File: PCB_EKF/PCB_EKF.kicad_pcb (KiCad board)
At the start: 2 copper layers, 97.8 x 84.6 mm, 41 parts, among them J1 Load, J2 5V, J4 UART, K1 SANYOU_SRD_Form_C, K3 SANYOU_SRD_Form_C, Q1 Q_NMOS_GSD, Q3 Q_NMOS_GSD, SW1 SW_Push_SPDT, U1 INA226_module, U3 YAAJ_BlackPill_Part_Like_SWD_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, U4 TP4056_Module, U5 AMS1117-3.3

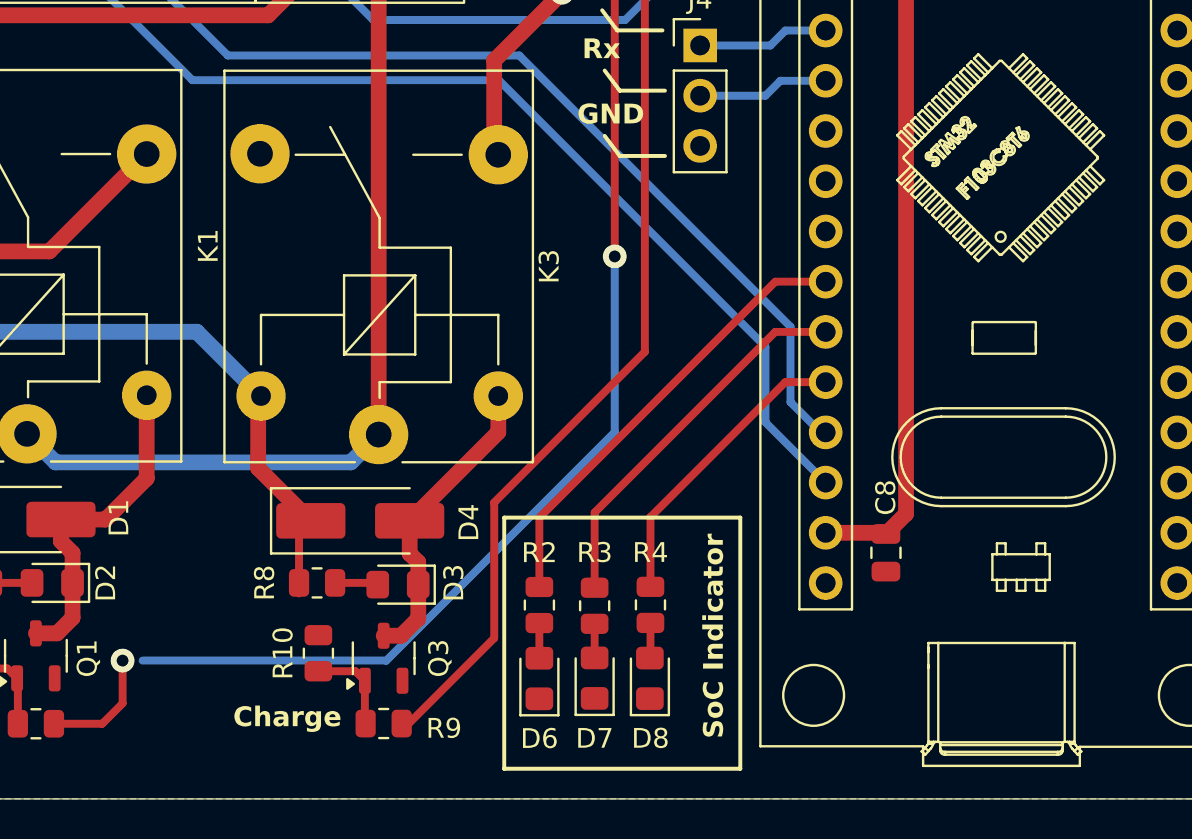
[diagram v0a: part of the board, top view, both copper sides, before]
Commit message: add a lot
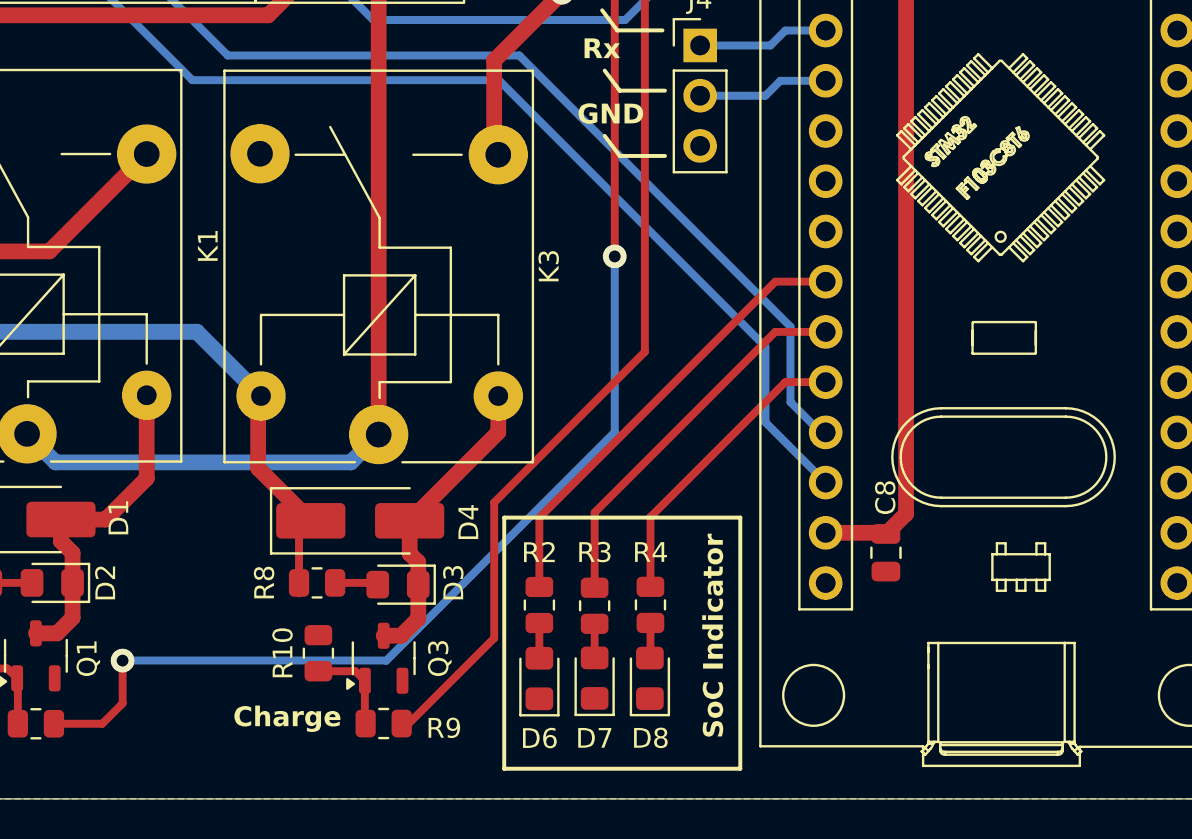
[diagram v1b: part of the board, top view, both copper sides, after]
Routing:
- net CTRL_Load: track 87.8 -> 88.8 mm
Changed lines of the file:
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@@
 			(outputformat 1)
 			(mirror no)
-			(drillshape 1)
+			(drillshape 0)
 			(scaleselection 1)
-			(outputdirectory "")
+			(outputdirectory "Gerber/")
 		)
 	)
@@
 		(fp_arc
 			(start 5.210659 19.015233)
-			(mid 5.273125 18.98719)
+			(mid 5.273123 18.987169)
 			(end 5.341329 18.993348)
 			(stroke
@@
 		(fp_arc
 			(start 6.981719 17.244173)
-			(mid 7.051919 17.214426)
+			(mid 7.051919 17.214488)
 			(end 7.121632 17.245341)
 			(stroke
@@
 		(fp_arc
 			(start 8.464456 19.37686)
-			(mid 8.346161 19.099702)
+			(mid 8.346155 19.099702)
 			(end 8.463393 18.822096)
 			(stroke
@@
 		(fp_arc
 			(start 8.924989 18.360501)
-			(mid 9.075715 18.294215)
+			(mid 9.075715 18.294151)
 			(end 9.227336 18.358376)
 			(stroke
@@
 		(fp_arc
 			(start 9.017838 18.458024)
-			(mid 9.077292 18.432027)
+			(mid 9.077292 18.432091)
 			(end 9.136717 18.458131)
 			(stroke
@@
 		(fp_arc
 			(start 11.989999 48.971818)
-			(mid 11.906797 49.125261)
+			(mid 11.906813 49.12524)
 			(end 11.739999 49.176605)
 			(stroke
@@
 		(fp_arc
 			(start 11.99 49.115212)
-			(mid 11.906844 49.268701)
+			(mid 11.906816 49.268638)
 			(end 11.739999 49.32)
 			(stroke
@@
 		(fp_arc
 			(start 12.464857 49.004759)
-			(mid 12.372292 48.850875)
+			(mid 12.372274 48.85088)
 			(end 12.340011 48.674215)
 			(stroke
@@
 		(fp_arc
 			(start 12.648833 48.840847)
-			(mid 12.603027 48.765284)
+			(mid 12.603045 48.765279)
 			(end 12.586427 48.6785)
 			(stroke
@@
 		)
 		(property "Value" "1k"
-			(at 0 1.65 360)
+			(at 0 1.65 0)
 			(layer "F.Fab")
 			(effects
@@
 		)
 		(fp_text user "${REFERENCE}"
-			(at 0 0 360)
+			(at 0 0 0)
 			(layer "F.Fab")
 			(effects
@@
 		(tags "resistor")
 		(property "Reference" "R9"
-			(at -3.048 -0.254 360)
+			(at -3.048 -0.254 0)
 			(layer "F.SilkS")
 			(effects
@@
 		)
 		(property "Value" "1k"
-			(at 0 1.65 360)
+			(at 0 1.65 0)
 			(layer "F.Fab")
 			(effects
@@
 		)
 		(fp_text user "${REFERENCE}"
-			(at 0 0 360)
+			(at 0 0 0)
 			(layer "F.Fab")
 			(effects
@@
 	(segment
 		(start 93.8605 105.2755)
-		(end 81.534 105.2755)
+		(end 80.5225 105.2755)
 		(width 0.4)
 		(layer "B.Cu")
